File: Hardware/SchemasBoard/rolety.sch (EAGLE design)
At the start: 29 parts, among them IC1 LNK304, IC2 MCP1703DB, K1 FRS1B, K2 FRS1B, T1 BC846, T2 BC846

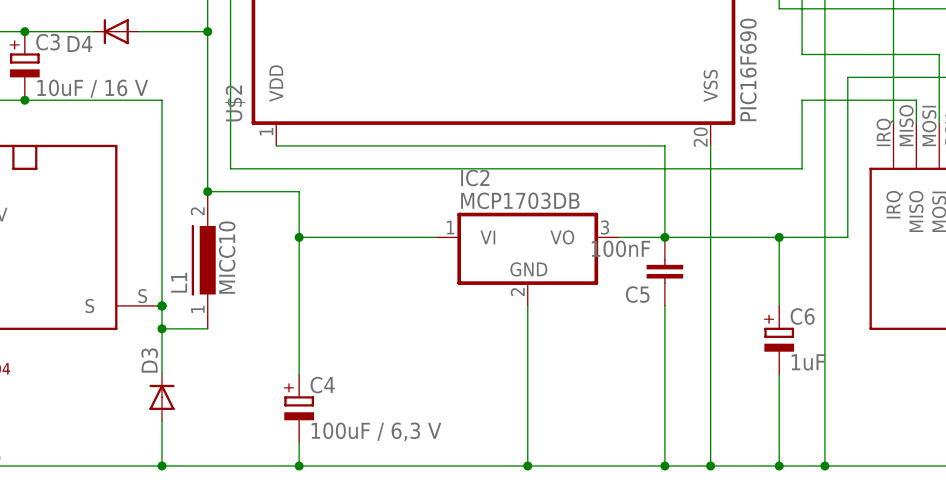
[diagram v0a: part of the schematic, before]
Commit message: hf
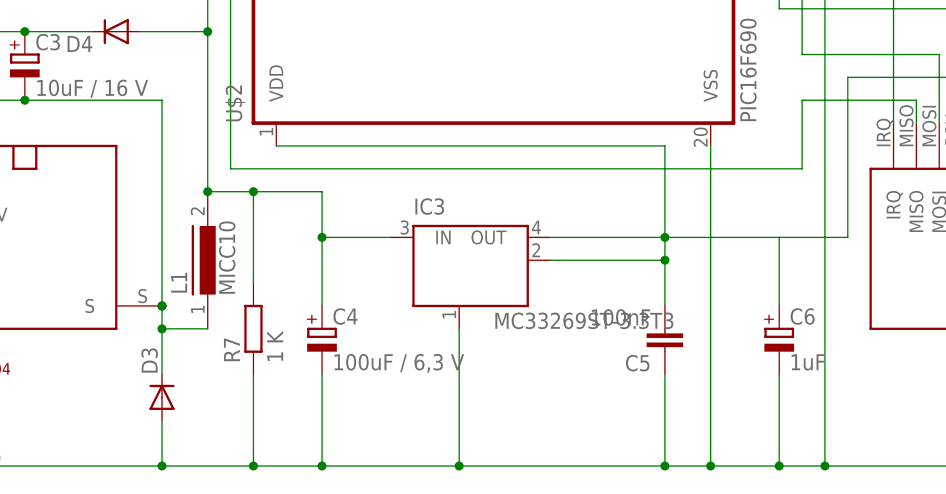
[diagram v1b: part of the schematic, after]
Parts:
- removed IC2: MCP1703DB, linear:MCP1703DB
- added IC3: MC33269ST-3.3T3, linear:MC33269ST-3.3T3
- added R7: 1 K, resistor:R-EU_M2012
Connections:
- net GND: now also IC3.GND/ADJ, R7.1; no longer IC2.GND
- net N$17: now also IC3.OUT, IC3.OUT@1; no longer IC2.VO
- net N$27: now also IC3.IN, R7.2; no longer IC2.VI
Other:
- moved on the sheet: C4, C5
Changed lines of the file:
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@@
 <part name="L1" library="inductors" deviceset="MICC10" device=""/>
 <part name="C4" library="resistor" deviceset="CPOL-EU" device="E2.5-5" value="100uF / 6,3 V"/>
-<part name="IC2" library="linear" deviceset="MCP1703" device="DB"/>
 <part name="C5" library="resistor" deviceset="C-EU" device="C2012" value="100nF"/>
 <part name="T1" library="transistor" deviceset="BC846" device=""/>
@@
 <part name="X1" library="con-ptr500" deviceset="AK500/4" device=""/>
 <part name="U$3" library="rfm70" deviceset="PROGRAMMINGHEADER" device="" technology="DIP"/>
+<part name="IC3" library="linear" deviceset="MC33269ST*" device="" technology="-3.3T3"/>
+<part name="R7" library="resistor" deviceset="R-EU_" device="M2012" value="1 K"/>
 </parts>
 <sheets>
@@
 <instance part="C3" gate="G$1" x="55.88" y="76.2"/>
 <instance part="L1" gate="1" x="76.2" y="53.34" rot="R90"/>
-<instance part="C4" gate="G$1" x="86.36" y="38.1"/>
-<instance part="IC2" gate="G$1" x="111.76" y="55.88"/>
-<instance part="C5" gate="G$1" x="127" y="50.8" rot="R180"/>
+<instance part="C4" gate="G$1" x="88.9" y="45.72"/>
+<instance part="C5" gate="G$1" x="127" y="43.18" rot="R180"/>
 <instance part="T1" gate="G$1" x="12.7" y="63.5" rot="R180"/>
 <instance part="D3" gate="G$1" x="71.12" y="38.1" rot="R90"/>
@@
 <instance part="X1" gate="-4" x="-38.1" y="48.26"/>
 <instance part="U$3" gate="G$1" x="177.8" y="134.62"/>
+<instance part="IC3" gate="G$1" x="104.14" y="50.8"/>
+<instance part="R7" gate="G$1" x="81.28" y="45.72" rot="R90"/>
 </instances>
 <busses>
@@
 <wire x1="20.32" y1="30.48" x2="22.86" y2="30.48" width="0.1524" layer="91"/>
 <wire x1="22.86" y1="30.48" x2="71.12" y2="30.48" width="0.1524" layer="91"/>
-<wire x1="71.12" y1="30.48" x2="86.36" y2="30.48" width="0.1524" layer="91"/>
-<wire x1="86.36" y1="30.48" x2="111.76" y2="30.48" width="0.1524" layer="91"/>
-<wire x1="111.76" y1="30.48" x2="127" y2="30.48" width="0.1524" layer="91"/>
+<wire x1="71.12" y1="30.48" x2="81.28" y2="30.48" width="0.1524" layer="91"/>
+<wire x1="81.28" y1="30.48" x2="88.9" y2="30.48" width="0.1524" layer="91"/>
+<wire x1="88.9" y1="30.48" x2="104.14" y2="30.48" width="0.1524" layer="91"/>
+<wire x1="104.14" y1="30.48" x2="127" y2="30.48" width="0.1524" layer="91"/>
 <wire x1="127" y1="30.48" x2="132.08" y2="30.48" width="0.1524" layer="91"/>
 <wire x1="132.08" y1="30.48" x2="139.7" y2="30.48" width="0.1524" layer="91"/>
@@
 <wire x1="71.12" y1="35.56" x2="71.12" y2="30.48" width="0.1524" layer="91"/>
 <junction x="71.12" y="30.48"/>
-<pinref part="IC2" gate="G$1" pin="GND"/>
-<wire x1="111.76" y1="48.26" x2="111.76" y2="30.48" width="0.1524" layer="91"/>
-<junction x="111.76" y="30.48"/>
 <pinref part="C5" gate="G$1" pin="1"/>
-<wire x1="127" y1="48.26" x2="127" y2="30.48" width="0.1524" layer="91"/>
+<wire x1="127" y1="40.64" x2="127" y2="30.48" width="0.1524" layer="91"/>
 <pinref part="U$2" gate="G$1" pin="VSS"/>
 <wire x1="132.08" y1="66.04" x2="132.08" y2="30.48" width="0.1524" layer="91"/>
@@
 <junction x="22.86" y="30.48"/>
 <pinref part="C4" gate="G$1" pin="-"/>
-<wire x1="86.36" y1="33.02" x2="86.36" y2="30.48" width="0.1524" layer="91"/>
-<junction x="86.36" y="30.48"/>
+<wire x1="88.9" y1="40.64" x2="88.9" y2="30.48" width="0.1524" layer="91"/>
+<junction x="88.9" y="30.48"/>
 <pinref part="D3" gate="G$1" pin="A"/>
 <wire x1="20.32" y1="121.92" x2="20.32" y2="68.58" width="0.1524" layer="91"/>
@@
 <wire x1="162.56" y1="134.62" x2="162.56" y2="119.38" width="0.1524" layer="91"/>
 <wire x1="162.56" y1="119.38" x2="177.8" y2="119.38" width="0.1524" layer="91"/>
+<pinref part="IC3" gate="G$1" pin="GND/ADJ"/>
+<wire x1="104.14" y1="45.72" x2="104.14" y2="30.48" width="0.1524" layer="91"/>
+<junction x="104.14" y="30.48"/>
+<pinref part="R7" gate="G$1" pin="1"/>
+<wire x1="81.28" y1="40.64" x2="81.28" y2="30.48" width="0.1524" layer="91"/>
+<junction x="81.28" y="30.48"/>
 </segment>
 </net>
@@
 <net name="N$17" class="0">
 <segment>
-<pinref part="C5" gate="G$1" pin="2"/>
-<pinref part="IC2" gate="G$1" pin="VO"/>
-<wire x1="127" y1="55.88" x2="121.92" y2="55.88" width="0.1524" layer="91"/>
-<pinref part="U$2" gate="G$1" pin="VDD"/>
-<wire x1="83.82" y1="66.04" x2="127" y2="66.04" width="0.1524" layer="91"/>
-<wire x1="127" y1="66.04" x2="127" y2="55.88" width="0.1524" layer="91"/>
-<junction x="127" y="55.88"/>
-<wire x1="127" y1="55.88" x2="139.7" y2="55.88" width="0.1524" layer="91"/>
 <wire x1="139.7" y1="55.88" x2="147.32" y2="55.88" width="0.1524" layer="91"/>
 <wire x1="147.32" y1="55.88" x2="147.32" y2="73.66" width="0.1524" layer="91"/>
@@
 <pinref part="C6" gate="G$1" pin="+"/>
 <wire x1="139.7" y1="48.26" x2="139.7" y2="55.88" width="0.1524" layer="91"/>
-<junction x="139.7" y="55.88"/>
 <pinref part="U$3" gate="G$1" pin="VDD"/>
 <wire x1="160.02" y1="132.08" x2="167.64" y2="132.08" width="0.1524" layer="91"/>
+<pinref part="C5" gate="G$1" pin="2"/>
+<wire x1="127" y1="66.04" x2="127" y2="55.88" width="0.1524" layer="91"/>
+<pinref part="U$2" gate="G$1" pin="VDD"/>
+<wire x1="127" y1="55.88" x2="127" y2="53.34" width="0.1524" layer="91"/>
+<wire x1="127" y1="53.34" x2="127" y2="48.26" width="0.1524" layer="91"/>
+<wire x1="83.82" y1="66.04" x2="127" y2="66.04" width="0.1524" layer="91"/>
+<wire x1="139.7" y1="55.88" x2="127" y2="55.88" width="0.1524" layer="91"/>
+<junction x="127" y="55.88"/>
+<pinref part="IC3" gate="G$1" pin="OUT"/>
+<wire x1="114.3" y1="55.88" x2="127" y2="55.88" width="0.1524" layer="91"/>
+<pinref part="IC3" gate="G$1" pin="OUT@1"/>
+<wire x1="114.3" y1="53.34" x2="127" y2="53.34" width="0.1524" layer="91"/>
+<junction x="127" y="53.34"/>
 </segment>
 </net>
@@
 <wire x1="33.02" y1="83.82" x2="76.2" y2="83.82" width="0.1524" layer="91"/>
 <wire x1="0" y1="81.28" x2="0" y2="83.82" width="0.1524" layer="91"/>
-<pinref part="IC2" gate="G$1" pin="VI"/>
-<wire x1="101.6" y1="55.88" x2="86.36" y2="55.88" width="0.1524" layer="91"/>
-<wire x1="76.2" y1="60.96" x2="86.36" y2="60.96" width="0.1524" layer="91"/>
-<wire x1="86.36" y1="60.96" x2="86.36" y2="55.88" width="0.1524" layer="91"/>
+<wire x1="96.52" y1="55.88" x2="88.9" y2="55.88" width="0.1524" layer="91"/>
+<wire x1="76.2" y1="60.96" x2="81.28" y2="60.96" width="0.1524" layer="91"/>
+<wire x1="81.28" y1="60.96" x2="88.9" y2="60.96" width="0.1524" layer="91"/>
+<wire x1="88.9" y1="60.96" x2="88.9" y2="55.88" width="0.1524" layer="91"/>
 <junction x="76.2" y="60.96"/>
 <pinref part="C4" gate="G$1" pin="+"/>
-<wire x1="86.36" y1="40.64" x2="86.36" y2="55.88" width="0.1524" layer="91"/>
-<junction x="86.36" y="55.88"/>
+<wire x1="88.9" y1="48.26" x2="88.9" y2="55.88" width="0.1524" layer="91"/>
+<junction x="88.9" y="55.88"/>
 <pinref part="D4" gate="G$1" pin="A"/>
 <pinref part="D1" gate="G$1" pin="C"/>
@@
 <junction x="10.16" y="99.06"/>
 <junction x="0" y="99.06"/>
-</segment>
-</net>
+<pinref part="IC3" gate="G$1" pin="IN"/>
+<pinref part="R7" gate="G$1" pin="2"/>
+<wire x1="81.28" y1="50.8" x2="81.28" y2="60.96" width="0.1524" layer="91"/>
+<junction x="81.28" y="60.96"/>
+</segment>
+</net>
